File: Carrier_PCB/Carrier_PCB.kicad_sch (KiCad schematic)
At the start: 39 parts, among them J1 Conn_01x24, J2 Conn_01x24

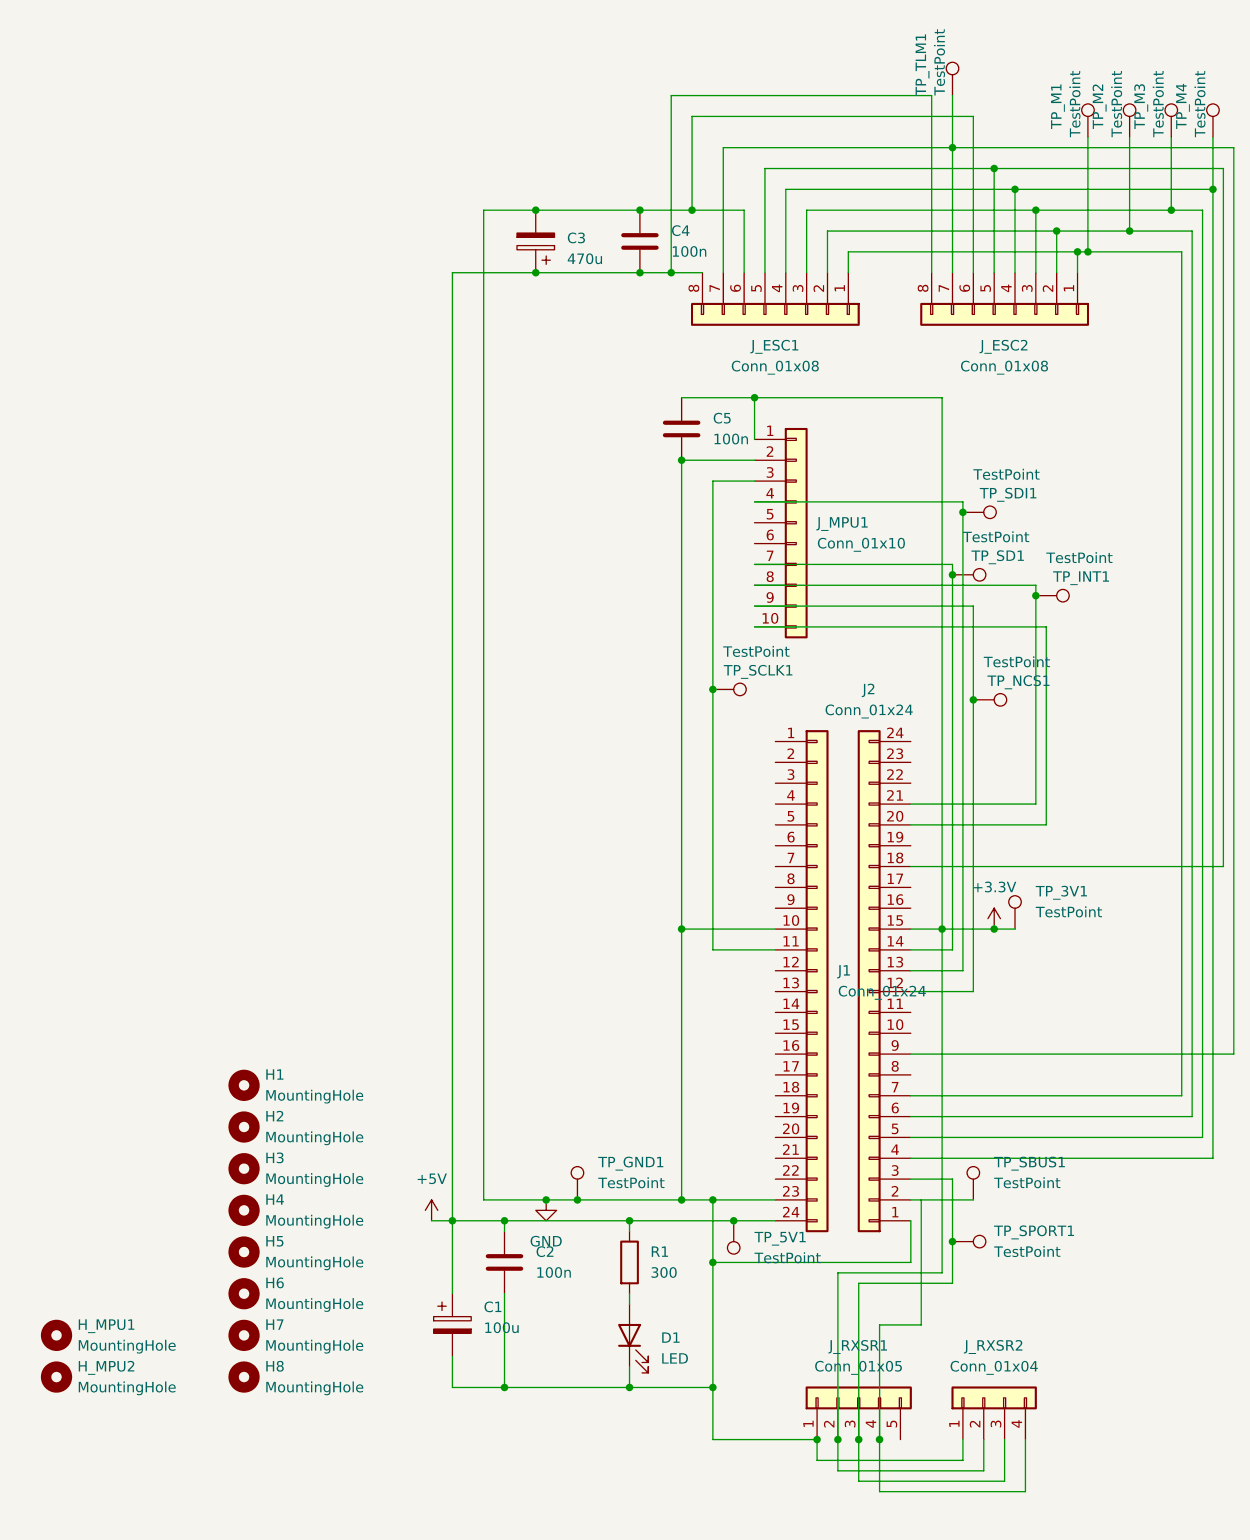
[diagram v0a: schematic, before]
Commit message: Update PCB. Not wired yet
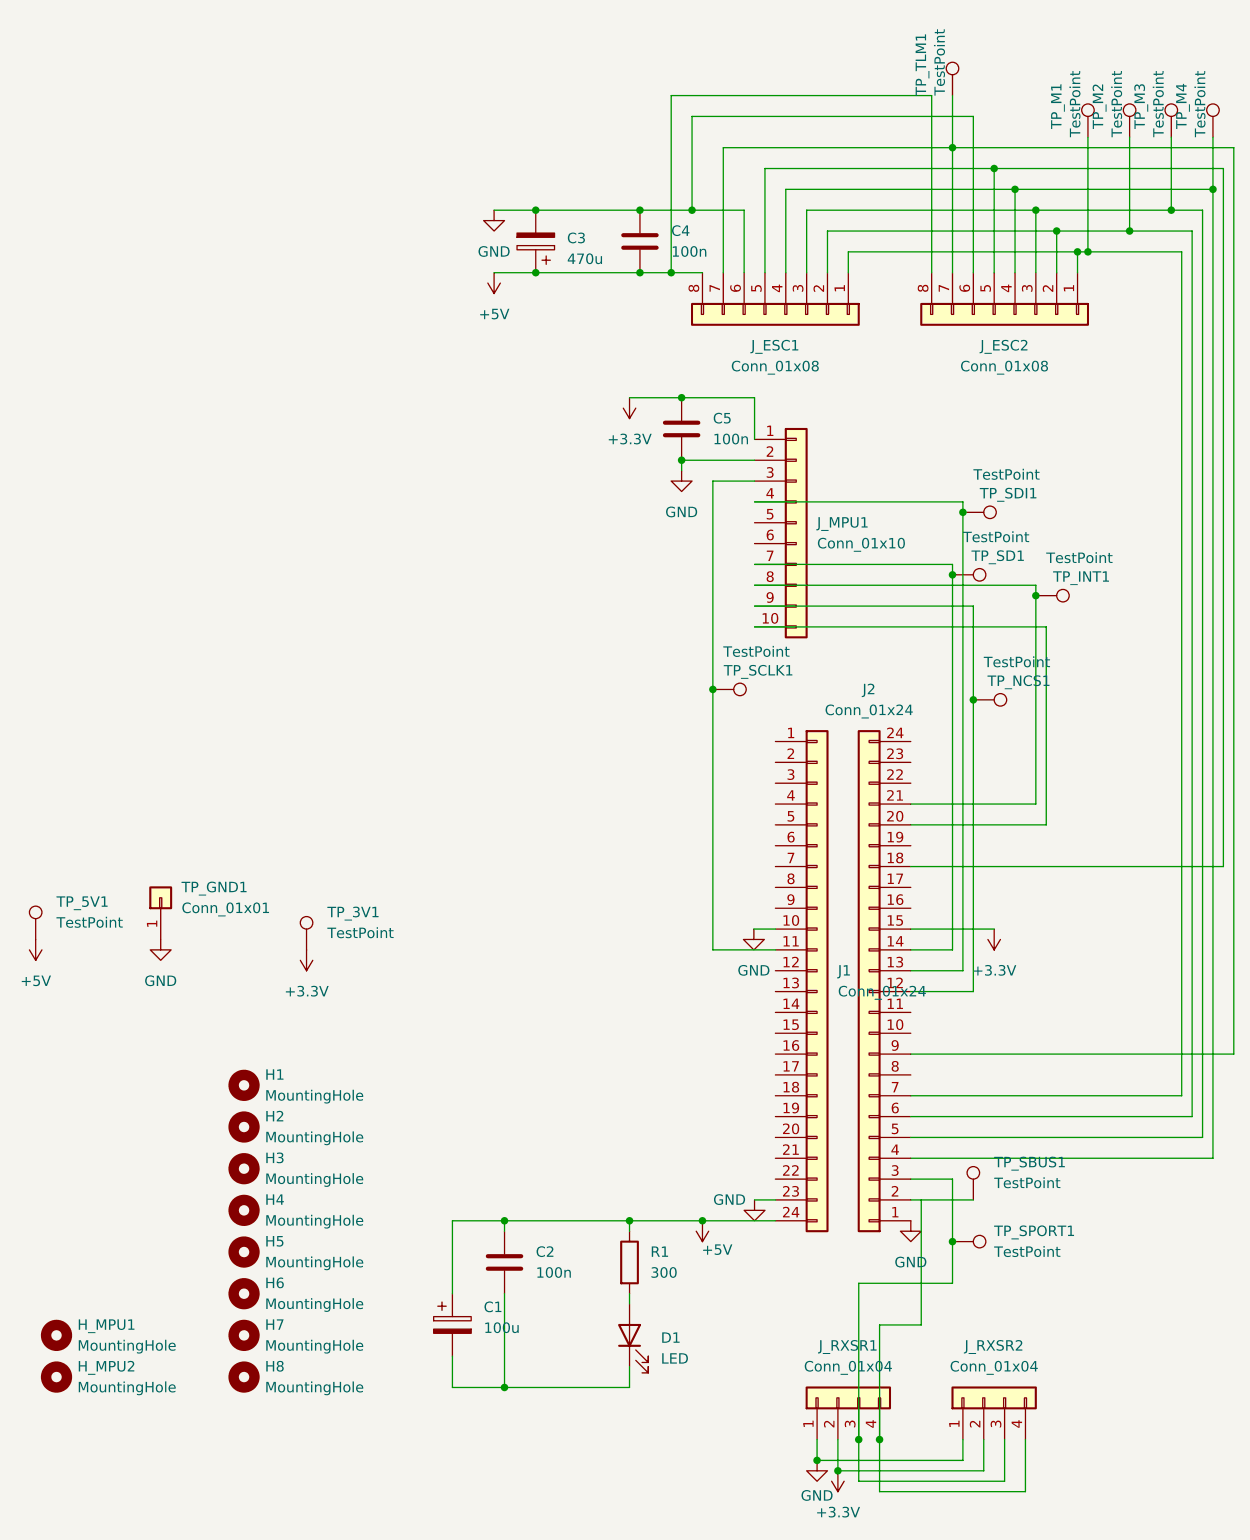
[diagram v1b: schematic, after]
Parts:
- removed J_RXSR1: Conn_01x05, Connector_PinSocket_2.54mm:PinSocket_1x05_P2.54mm_Horizontal, symbol Connector_Generic:Conn_01x05
- removed TP_GND1: TestPoint, TestPoint:TestPoint_Bridge_Pitch2.54mm_Drill0.7mm, symbol Connector:TestPoint
- added J_RXSR1: Conn_01x04, Connector_PinHeader_2.54mm:PinHeader_1x04_P2.54mm_Horizontal, symbol Connector_Generic:Conn_01x04
- added TP_GND1: Conn_01x01, Connector_PinHeader_2.54mm:PinHeader_1x01_P2.54mm_Horizontal, symbol Connector_Generic:Conn_01x01
- J_ESC1: footprint Connector_PinSocket_2.54mm:PinSocket_1x08_P2.54mm_Horizontal -> Connector_PinHeader_2.54mm:PinHeader_1x08_P2.54mm_Horizontal
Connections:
- net +3.3V: now also J_RXSR1.2 (Pin_2)
- net GND: now also J_RXSR1.1 (Pin_1), TP_GND1.1 (Pin_1); no longer C1.2, C2.2, D1.1 (K)
- net at J2.3 (Pin_3), J_RXSR2.3 (Pin_3), TP_SPORT1.1: now also J_RXSR1.3 (Pin_3)
- net at J_RXSR2.4 (Pin_4): now also J_RXSR1.4 (Pin_4)
- new net: C1.2, C2.2, D1.1 (K)
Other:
- moved on the sheet: TP_3V1, TP_5V1
